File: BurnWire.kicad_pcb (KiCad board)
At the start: 2 copper layers, 14 parts, among them J1 B6B-XH-A_LF__SN_, U1 ADP2303ARDZ

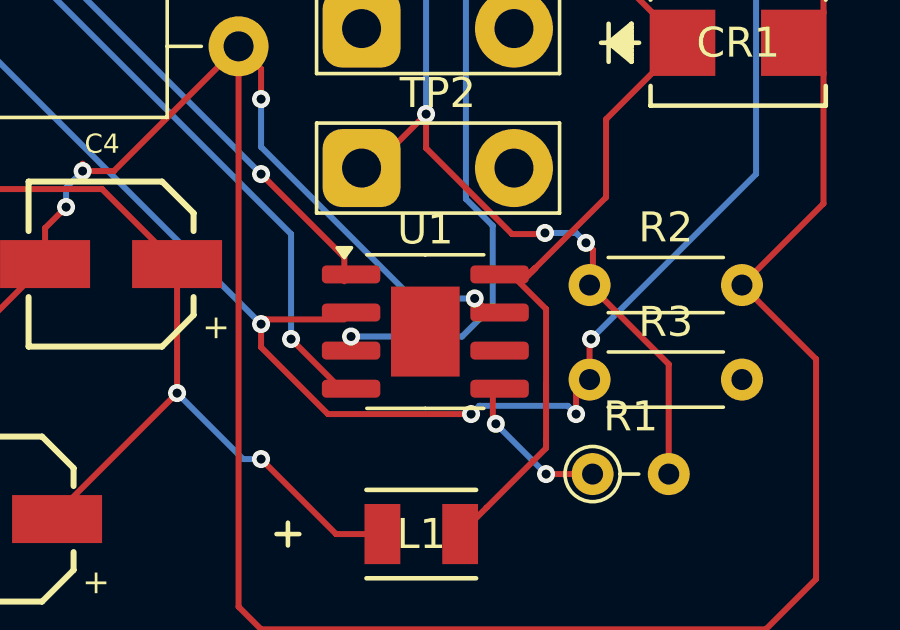
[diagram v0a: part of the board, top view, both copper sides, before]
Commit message: done
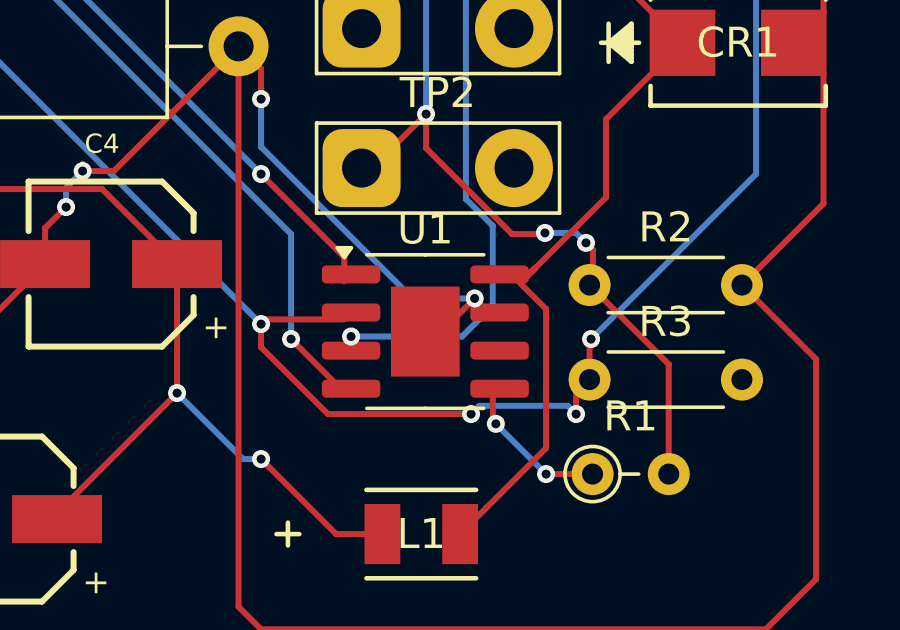
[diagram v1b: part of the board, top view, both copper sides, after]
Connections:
- U1 pad 9: unconnected-(U1-PADGND-Pad9) -> GND
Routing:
- net GND: track 118.4 -> 120.5 mm
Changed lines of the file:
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@@
 			(psa4output no)
 			(plot_black_and_white yes)
-			(sketchpadsonfab no)
+			(sketchpadsonfab yes)
 			(plotpadnumbers no)
 			(hidednponfab no)
 			(sketchdnponfab yes)
 			(crossoutdnponfab yes)
-			(subtractmaskfromsilk no)
+			(subtractmaskfromsilk yes)
 			(outputformat 1)
 			(mirror no)
-			(drillshape 1)
+			(drillshape 0)
 			(scaleselection 1)
-			(outputdirectory "")
+			(outputdirectory "gerber/")
 		)
 	)
@@
 	(net 9 "Net-(U1-FB)")
 	(net 10 "unconnected-(U1-NC-Pad6)")
-	(net 11 "unconnected-(U1-PADGND-Pad9)")
 	(footprint "TestPoint:TestPoint_2Pads_Pitch5.08mm_Drill1.3mm"
 		(layer "F.Cu")
@@
 			(property pad_prop_heatsink)
 			(layers "F.Cu" "F.Mask")
-			(net 11 "unconnected-(U1-PADGND-Pad9)")
+			(net 3 "GND")
 			(pinfunction "PADGND")
 			(pintype "power_in")
@@
 	)
 	(segment
-		(start 155.951 89.549)
-		(end 162.9743 89.549)
+		(start 160.5 103.5)
+		(end 160.5 103)
 		(width 0.2)
 		(layer "F.Cu")
@@
 	)
 	(segment
-		(start 160.5 103.5)
-		(end 160.5 103)
+		(start 160.1375 99.1375)
+		(end 159.699999 99.575)
 		(width 0.2)
 		(layer "F.Cu")
@@
 	)
 	(segment
-		(start 160.1375 99.1375)
-		(end 159.699999 99.575)
+		(start 162.9743 89.549)
+		(end 165.049 91.6237)
 		(width 0.2)
 		(layer "F.Cu")
@@
 	)
 	(segment
-		(start 154.35 91.15)
-		(end 155.951 89.549)
-		(width 0.2)
-		(layer "F.Cu")
-		(net 1)
-	)
-	(segment
-		(start 162.9743 89.549)
-		(end 165.049 91.6237)
-		(width 0.2)
-		(layer "F.Cu")
-		(net 1)
-	)
-	(segment
 		(start 157.63525 108)
 		(end 158.515 107.12025)
@@
 	)
 	(segment
+		(start 154.35 91.15)
+		(end 155.951 89.549)
+		(width 0.2)
+		(layer "F.Cu")
+		(net 1)
+	)
+	(segment
 		(start 159.8875 99.3875)
 		(end 158.9925 99.3875)
@@
 	)
 	(segment
+		(start 155.951 89.549)
+		(end 162.9743 89.549)
+		(width 0.2)
+		(layer "F.Cu")
+		(net 1)
+	)
+	(segment
 		(start 162.5 94.1727)
 		(end 162.5 96.774999)
@@
 	)
 	(segment
+		(start 157.015002 101.25)
+		(end 158.120002 100.145)
+		(width 0.2)
+		(layer "F.Cu")
+		(net 3)
+	)
+	(segment
 		(start 168.7574 91.6237)
 		(end 169.7474 90.6337)
@@
 		(width 0.2)
 		(layer "F.Cu")
+		(net 3)
+	)
+	(segment
+		(start 156.475 101.25)
+		(end 157.015002 101.25)
+		(width 0.2)
+		(layer "F.Cu")
